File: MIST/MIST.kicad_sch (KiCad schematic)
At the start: 2 parts, among them J1 Conn_01x08, J2 Conn_01x08

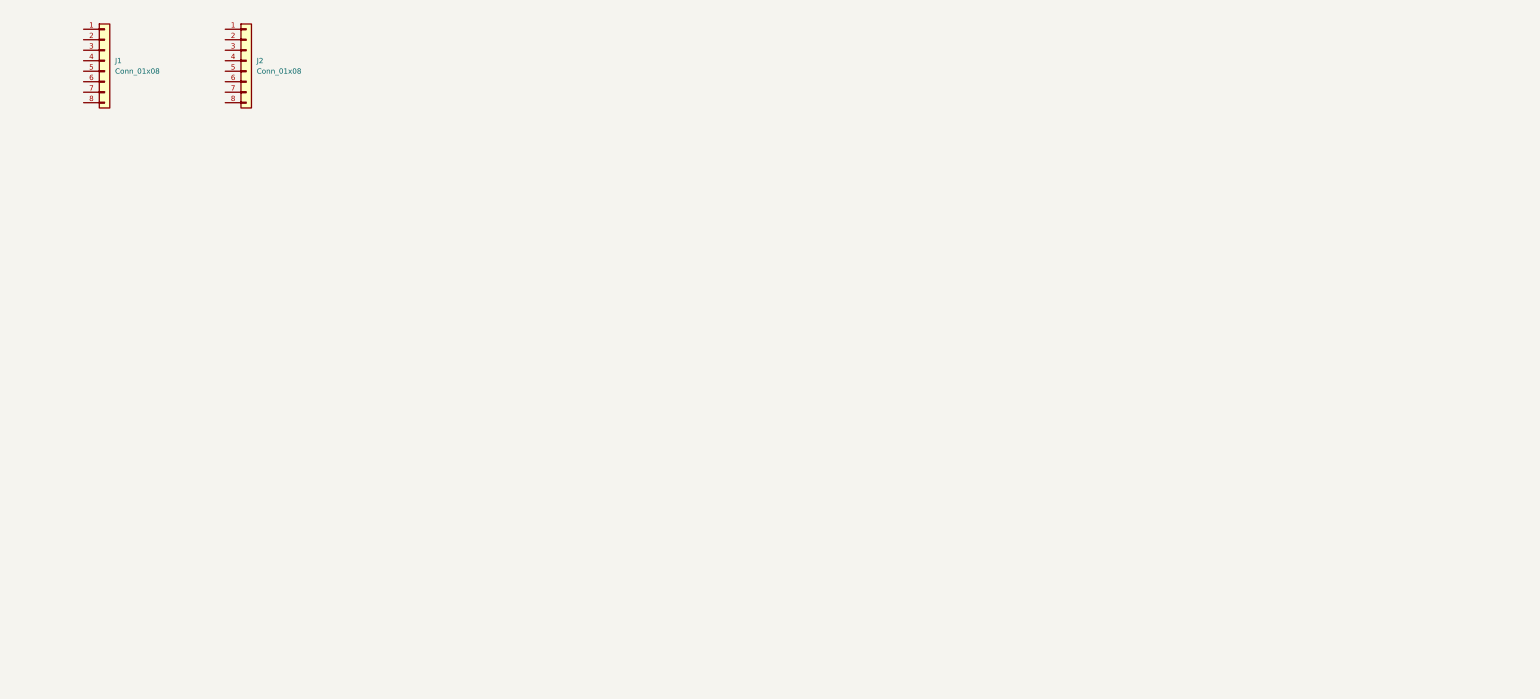
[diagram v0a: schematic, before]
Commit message: finished schematic. updated BOM. stuff.
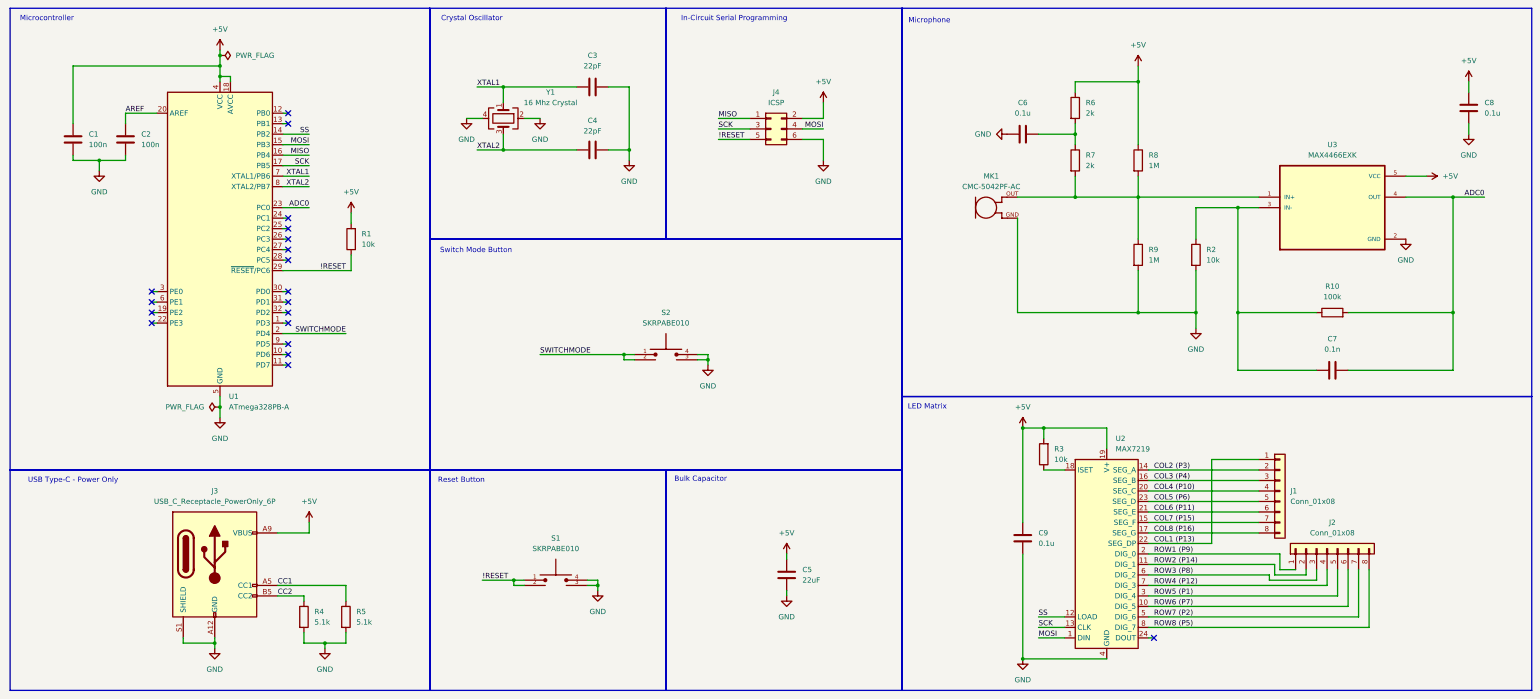
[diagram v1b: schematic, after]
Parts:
- added C1, C2: 100n, Capacitor_SMD:C_0805_2012Metric, symbol Device:C
- added C3, C4: 22pF, Capacitor_SMD:C_0805_2012Metric, symbol Device:C
- added C5: 22uF, Capacitor_SMD:C_0805_2012Metric, symbol Device:C
- added C6, C8, C9: 0.1u, symbol Device:C
- added C7: 0.1n, symbol Device:C
- added J3: USB_C_Receptacle_PowerOnly_6P, Connector_USB:USB_C_Receptacle_GCT_USB4125-xx-x_6P_TopMnt_Horizontal, symbol Connector:USB_C_Receptacle_PowerOnly_6P
- added J4: ICSP, Connector_PinHeader_2.54mm:PinHeader_2x03_P2.54mm_Vertical, symbol Connector_Generic:Conn_02x03_Odd_Even
- added MK1: CMC-5042PF-AC, CMC-5042PF-AC:CUI_CMC-5042PF-AC, symbol CMC-5042PF-AC:CMC-5042PF-AC
- added R1: 10k, Resistor_SMD:R_1206_3216Metric, symbol Device:R
- added R10: 100k, symbol Device:R
- added R2, R3: 10k, symbol Device:R
- added R4, R5: 5.1k, Resistor_SMD:R_1206_3216Metric, symbol Device:R
- added R6, R7: 2k, symbol Device:R
- added R8, R9: 1M, symbol Device:R
- added S1, S2: SKRPABE010, SKRPABE010:SW_SKRPABE010, symbol SKRPABE010:SKRPABE010
- added U1: ATmega328PB-A, Package_QFP:TQFP-32_7x7mm_P0.8mm, symbol MCU_Microchip_ATmega:ATmega328PB-A
- added U2: MAX7219, symbol Driver_LED:MAX7219
- added U3: MAX4466EXK, MAX4466EXK:SOT65P210X110-5N, symbol MAX4466EXK:MAX4466EXK
- added Y1: 16 Mhz Crystal, Crystal:Crystal_SMD_3225-4Pin_3.2x2.5mm, symbol Device:Crystal_GND24
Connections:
- net ROW1 (P9): now reaches J2.1 (Pin_1)
- net ROW1 (P9): now also U2.2 (DIG_0)
- net ROW2 (P14): now reaches J2.2 (Pin_2)
- net ROW2 (P14): now also U2.11 (DIG_1)
- net ROW3 (P8): now reaches J2.3 (Pin_3)
- net ROW3 (P8): now also U2.6 (DIG_2)
- net ROW4 (P12): now reaches J2.4 (Pin_4)
- net ROW4 (P12): now also U2.7 (DIG_3)
- net ROW5 (P1): now reaches J2.5 (Pin_5)
- net ROW5 (P1): now also U2.3 (DIG_4)
- net ROW6 (P7): now reaches J2.6 (Pin_6)
- net ROW6 (P7): now also U2.10 (DIG_5)
- net ROW7 (P2): now reaches J2.7 (Pin_7)
- net ROW7 (P2): now also U2.5 (DIG_6)
- net ROW8 (P5): now reaches J2.8 (Pin_8)
- net ROW8 (P5): now also U2.8 (DIG_7)
- net COL1 (P13): now reaches J1.1 (Pin_1)
- net COL1 (P13): now also U2.22 (SEG_DP)
- net COL2 (P3): now reaches J1.2 (Pin_2)
- net COL2 (P3): now also U2.14 (SEG_A)
- net COL3 (P4): now reaches J1.3 (Pin_3)
- net COL3 (P4): now also U2.16 (SEG_B)
- net COL4 (P10): now reaches J1.4 (Pin_4)
- net COL4 (P10): now also U2.20 (SEG_C)
- net COL5 (P6): now reaches J1.5 (Pin_5)
- net COL5 (P6): now also U2.23 (SEG_D)
- net COL6 (P11): now reaches J1.6 (Pin_6)
- net COL6 (P11): now also U2.21 (SEG_E)
- net COL7 (P15): now reaches J1.7 (Pin_7)
- net COL7 (P15): now also U2.15 (SEG_F)
- net COL8 (P16): now reaches J1.8 (Pin_8)
- net COL8 (P16): now also U2.17 (SEG_G)
- new net: C6.2, R6.2, R7.1
- new net: MK1.OUT, R7.2, R8.2, R9.1, U3.1 (IN+)
- new net: R3.1, U2.18 (ISET)
- new net: C7.1, R10.1, R2.1, U3.3 (IN-)
- new net !RESET: J4.5 (Pin_5), R1.1, S1.1, S1.2, U1.29 (~{RESET}/PC6)
- new net +5V: C1.2, C5.2, C8.1, C9.1, J3.A9 (VBUS), J3.B9 (VBUS), J4.2 (Pin_2), R1.2, R3.2, R6.1, R8.1, U1.18 (AVCC), U1.4 (VCC), U2.19 (V+), U3.5 (VCC)
- new net ADC0: C7.2, R10.2, U1.23 (PC0), U3.4 (OUT)
- new net AREF: C2.2, U1.20 (AREF)
- new net CC1: J3.A5 (CC1), R5.1
- new net CC2: J3.B5 (CC2), R4.1
- new net GND: C1.1, C2.1, C3.2, C4.1, C5.1, C6.1, C8.2, C9.2, J3.A12 (GND), J3.B12 (GND), J3.S1 (SHIELD), J4.6 (Pin_6), MK1.GND, R2.2, R4.2, R5.2, R9.2, S1.3, S1.4, S2.3, S2.4, U1.21 (GND), U1.5 (GND), U2.4 (GND), U2.9 (GND), U3.2 (GND), Y1.2, Y1.4
- new net MISO: J4.1 (Pin_1), U1.16 (PB4)
- new net MOSI: J4.4 (Pin_4), U1.15 (PB3), U2.1 (DIN)
- new net SCK: J4.3 (Pin_3), U1.17 (PB5), U2.13 (CLK)
- new net SS: U1.14 (PB2), U2.12 (LOAD)
- new net SWITCHMODE: S2.1, S2.2, U1.2 (PD4)
- new net XTAL1: C3.1, U1.7 (XTAL1/PB6), Y1.1
- new net XTAL2: C4.2, U1.8 (XTAL2/PB7), Y1.3
- no-connect marks 0 -> 19
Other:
- note added: "Bulk Capacitor"
- note added: "Crystal Oscillator"
- note added: "In-Circuit Serial Programming"
- note added: "LED Matrix"
- note added: "Microcontroller"
- note added: "Microphone"
- note added: "Reset Button"
- note added: "Switch Mode Button"
- note added: "USB Type-C - Power Only"
- moved on the sheet: J1, J2

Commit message: finished schematic and layout
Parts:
- C6, C7, C8, C9, R3: footprint (none) -> Capacitor_SMD:C_0805_2012Metric
- R10, R2, R6, R7, R8, R9: footprint (none) -> Resistor_SMD:R_0805_2012Metric
- R4, R5: footprint Resistor_SMD:R_1206_3216Metric -> Capacitor_SMD:C_0805_2012Metric
- U2: footprint (none) -> Package_SO:SOIC-24W_7.5x15.4mm_P1.27mm
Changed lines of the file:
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@@
 			)
 		)
-		(property "Footprint" ""
+		(property "Footprint" "Capacitor_SMD:C_0805_2012Metric"
 			(at 266.7 48.5648 0)
 			(effects
@@
 			)
 		)
-		(property "Footprint" "Resistor_SMD:R_1206_3216Metric"
+		(property "Footprint" "Capacitor_SMD:C_0805_2012Metric"
 			(at 87.122 166.37 90)
 			(effects
@@
 			)
 		)
-		(property "Footprint" ""
+		(property "Footprint" "Resistor_SMD:R_0805_2012Metric"
 			(at 289.052 55.88 90)
 			(effects
@@
 			)
 		)
-		(property "Footprint" ""
+		(property "Footprint" "Capacitor_SMD:C_0805_2012Metric"
 			(at 269.748 127 90)
 			(effects
@@
 			)
 		)
-		(property "Footprint" ""
+		(property "Footprint" "Package_SO:SOIC-24W_7.5x15.4mm_P1.27mm"
 			(at 281.94 149.86 0)
 			(effects
@@
 			)
 		)
-		(property "Footprint" "Resistor_SMD:R_1206_3216Metric"
+		(property "Footprint" "Capacitor_SMD:C_0805_2012Metric"
 			(at 97.282 166.37 90)
 			(effects
@@
 			)
 		)
-		(property "Footprint" ""
+		(property "Footprint" "Resistor_SMD:R_0805_2012Metric"
 			(at 337.82 94.488 90)
 			(effects
@@
 			)
 		)
-		(property "Footprint" ""
+		(property "Footprint" "Capacitor_SMD:C_0805_2012Metric"
 			(at 341.63 105.7148 0)
 			(effects
@@
 			)
 		)
-		(property "Footprint" ""
+		(property "Footprint" "Capacitor_SMD:C_0805_2012Metric"
 			(at 263.8552 151.13 0)
 			(effects
@@
 			)
 		)
-		(property "Footprint" ""
+		(property "Footprint" "Resistor_SMD:R_0805_2012Metric"
 			(at 273.812 55.88 90)
 			(effects
@@
 			)
 		)
-		(property "Footprint" ""
+		(property "Footprint" "Resistor_SMD:R_0805_2012Metric"
 			(at 289.052 78.74 90)
 			(effects
@@
 			)
 		)
-		(property "Footprint" ""
+		(property "Footprint" "Resistor_SMD:R_0805_2012Metric"
 			(at 273.812 43.18 90)
 			(effects
@@
 			)
 		)
-		(property "Footprint" ""
+		(property "Footprint" "Resistor_SMD:R_0805_2012Metric"
 			(at 303.022 78.74 90)
 			(effects
@@
 			)
 		)
-		(property "Footprint" ""
+		(property "Footprint" "Capacitor_SMD:C_0805_2012Metric"
 			(at 371.8052 46.99 0)
 			(effects
